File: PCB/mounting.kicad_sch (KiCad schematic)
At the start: 26 parts

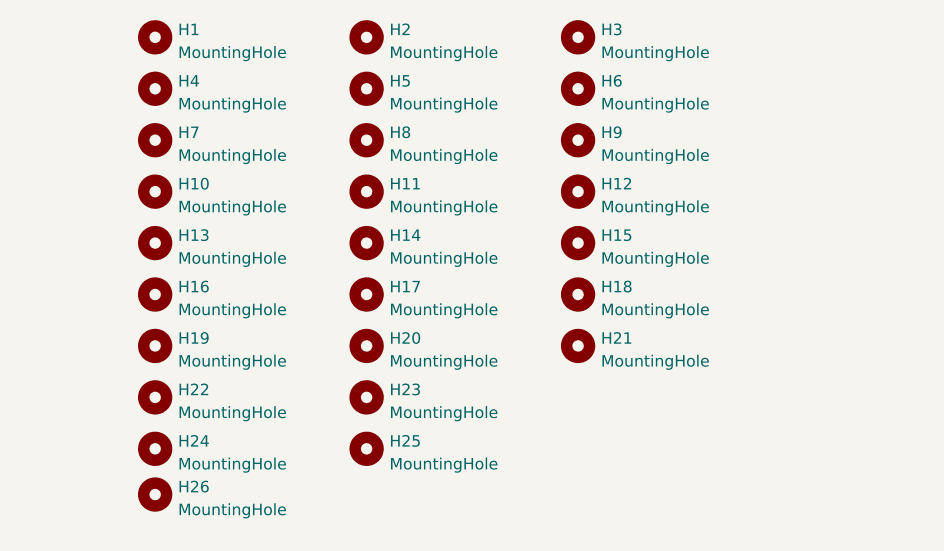
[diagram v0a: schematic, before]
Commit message: Update and pre-production output
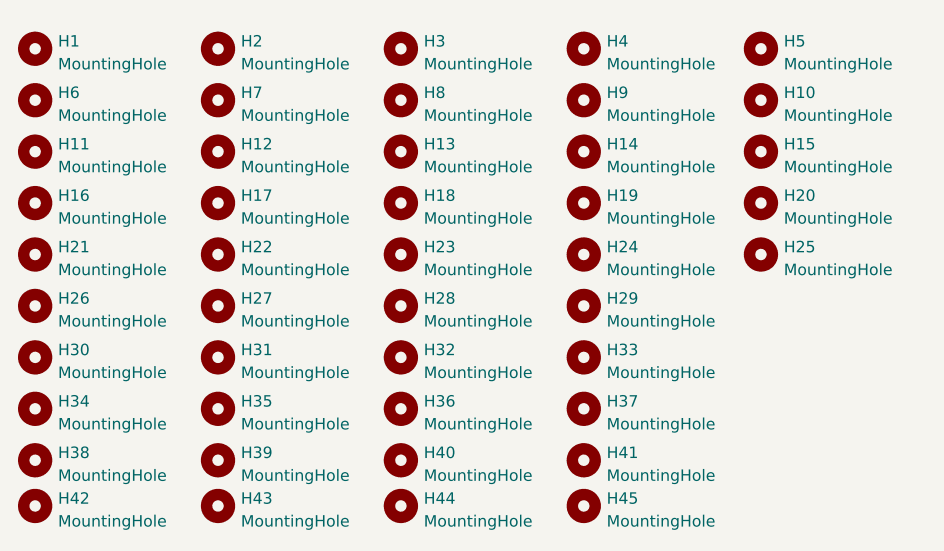
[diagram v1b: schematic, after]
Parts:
- removed H11, H21, H6: MountingHole, cipulot_parts:HOLE_M2_RF, symbol Mechanical:MountingHole
- added H10, H13, H19, H22, H24, H27, H28, H29, H31, H32, H33, H35, H36, H37, H39, H4, H40, H41, H43, H44, H45, H7: MountingHole, cipulot_parts:HOLE_M2_RF, symbol Mechanical:MountingHole
- renumbered H7 to H11, H10 to H16, H13 to H21, H16 to H26, H19 to H30, H22 to H34, H24 to H38, H26 to H42, H4 to H6
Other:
- moved on the sheet: H1, H11, H16, H21, H26, H30, H34, H38, H42, H6
